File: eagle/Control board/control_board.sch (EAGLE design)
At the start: 179 parts, among them SW1 SPST_TACT-EVQQ2, SW2 SPST_TACT-EVQQ2, U1 TCA9554A, U2 LM317, U3 LM317, U4 STM32F446, U5 TCA9554A, U6 TCA9554A, X1 JST-XH-02-PIN-LONG-PAD, X10 JST-XH-07-PIN-LONG-PAD, X11 JST-XH-07-PIN-LONG-PAD, X12 JST-XH-02-PIN-LONG-PAD, X13 JST-XH-03-PIN-LONG-PAD, X14 JST-XH-03-PIN-LONG-PAD, X15 JST-XH-08-PIN-LONG-PAD, X16 JST-XH-02-PIN-LONG-PAD, X17 JST-XH-08-PIN-LONG-PAD, X18 JST-XH-02-PIN-LONG-PAD, X2 JST-XH-06-PIN-LONG-PAD, X3 JST-XH-06-PIN-LONG-PAD, X4 JST-XH-06-PIN-LONG-PAD, X5 JST-XH-06-PIN-LONG-PAD, X6 JST-XH-06-PIN-LONG-PAD, X7 JST-XH-06-PIN-LONG-PAD, X8 JST-XH-04-PIN-LONG-PAD, X9 JST-XH-07-PIN-LONG-PAD

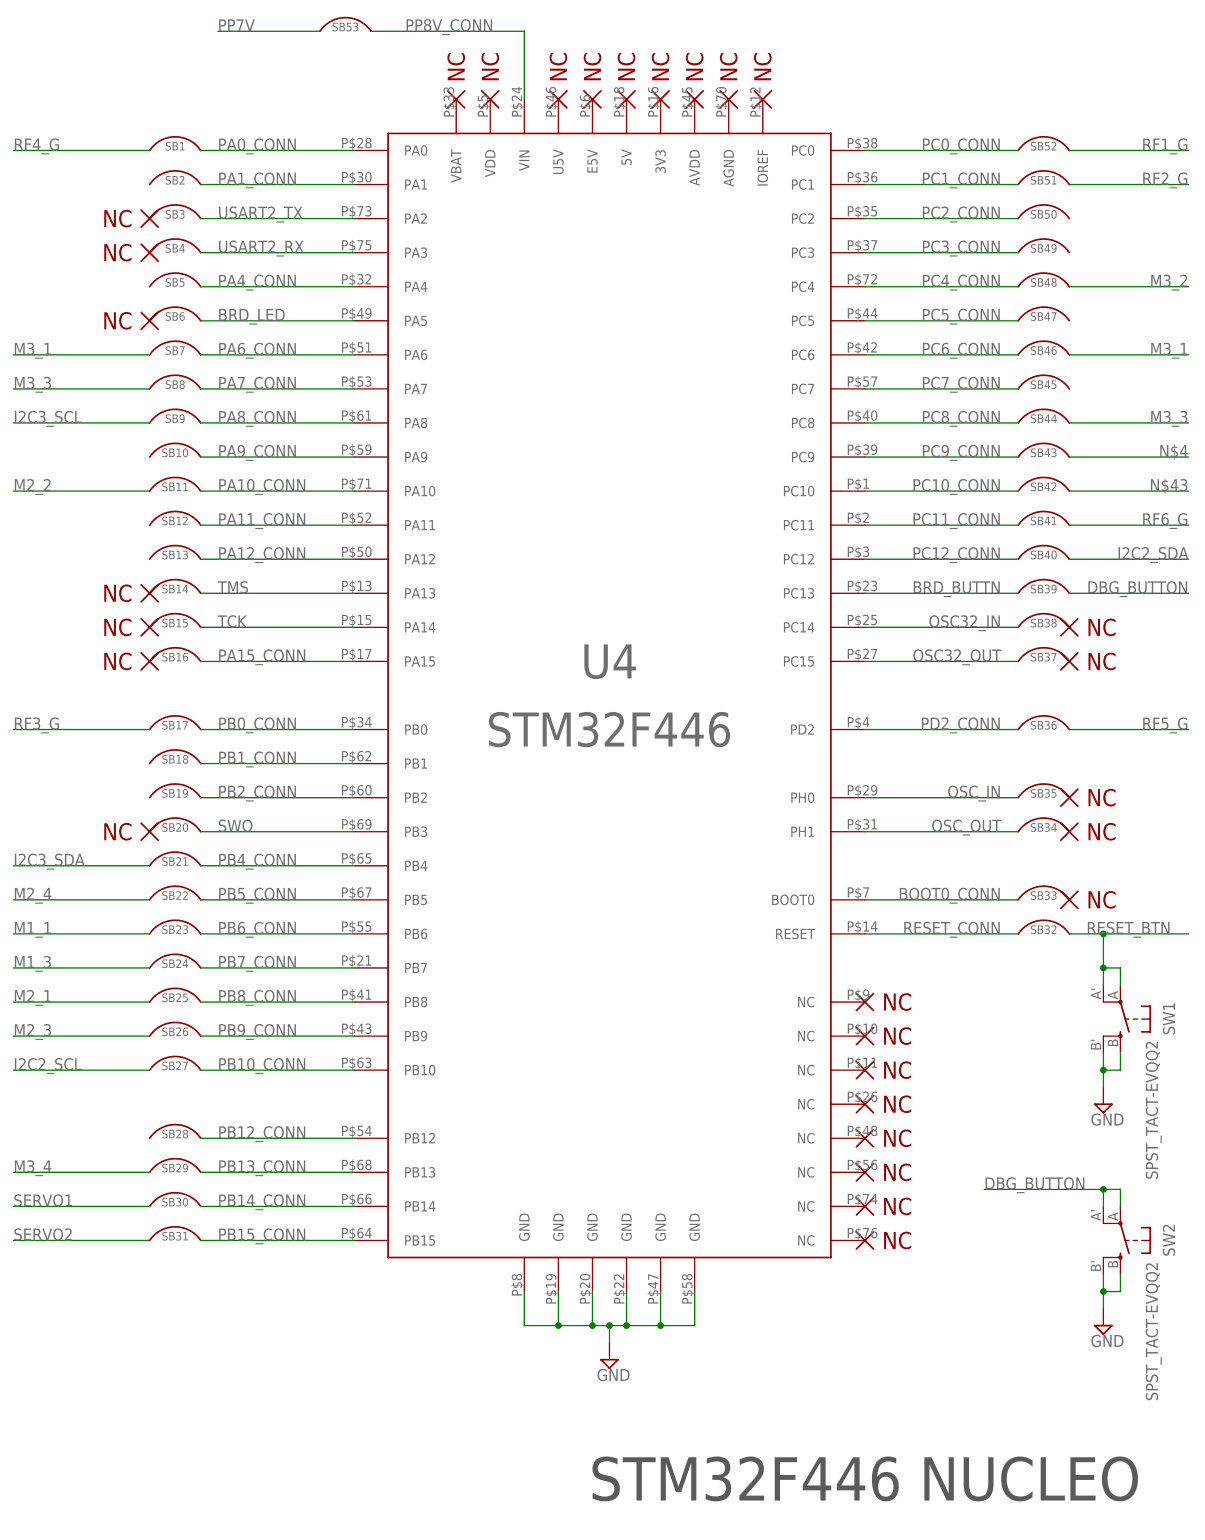
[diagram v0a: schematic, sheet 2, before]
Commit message: Nearly done assigning gpio
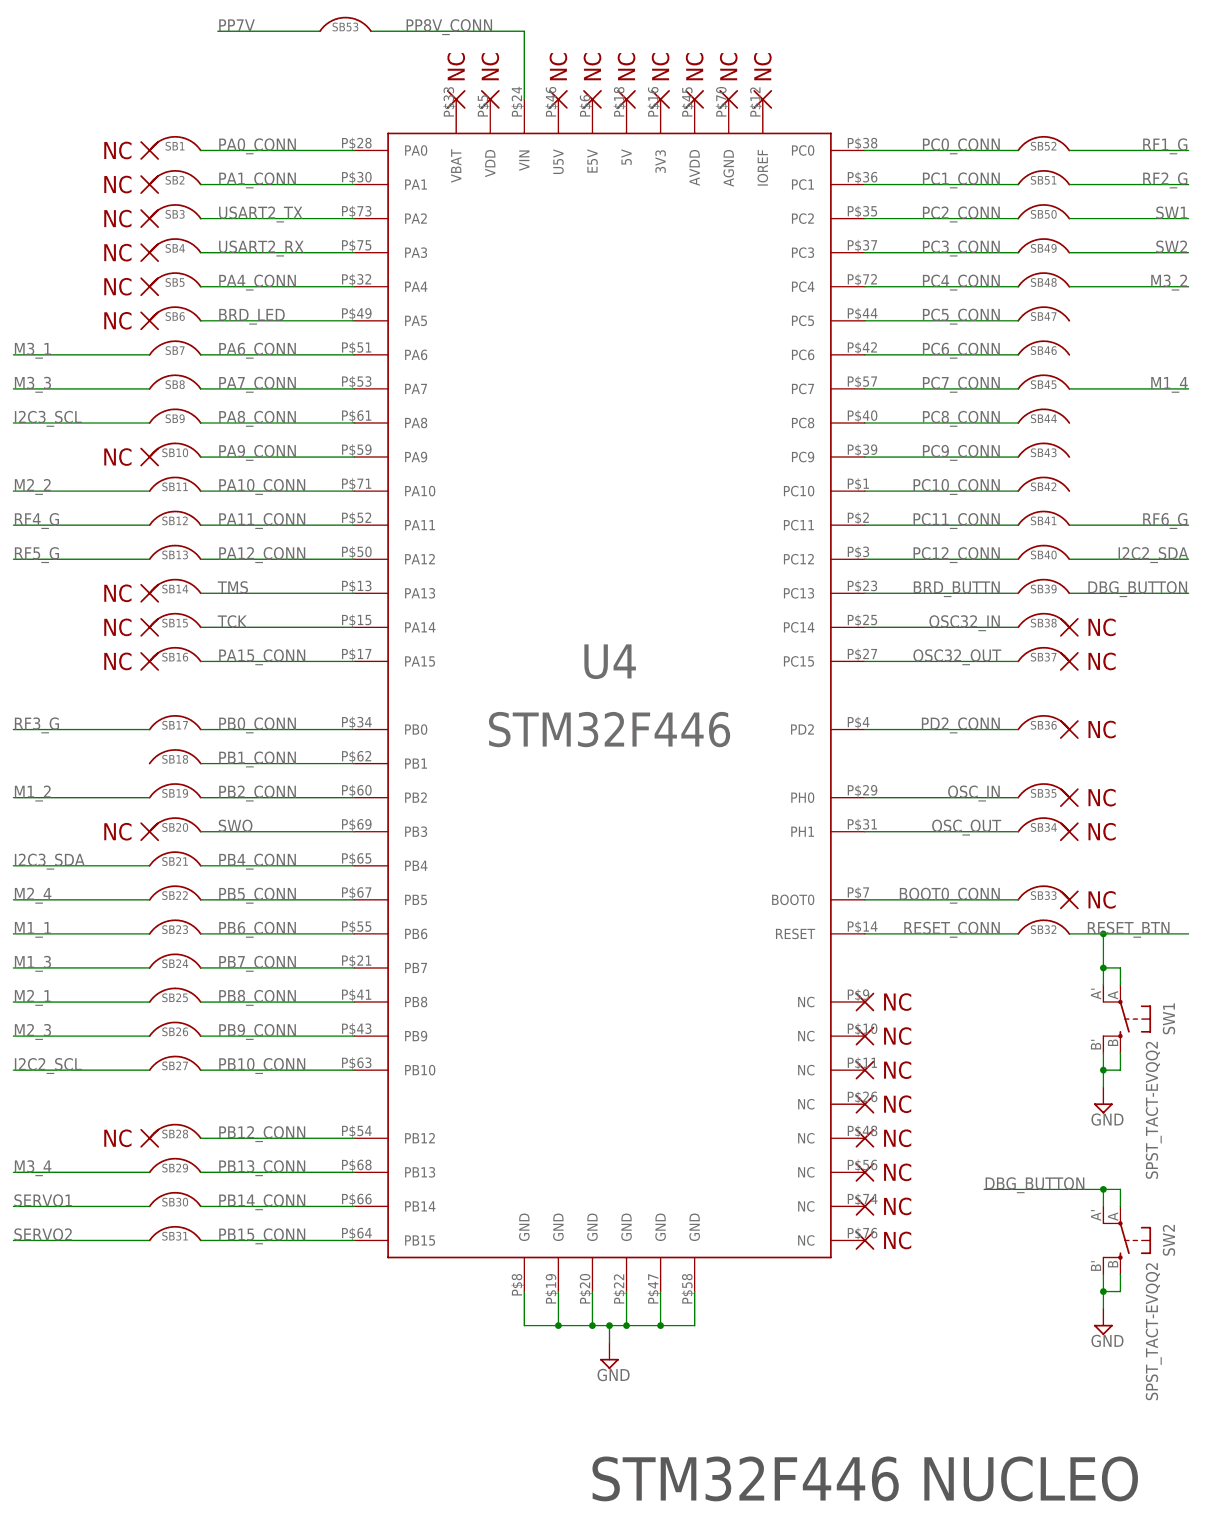
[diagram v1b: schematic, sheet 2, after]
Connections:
- removed net N$4: SB43.P$1
- removed net N$43: SB42.P$2
- net M1_2: now also SB19.P$1
- net M1_4: now also SB45.P$1
- net M3_1: no longer SB46.P$2
- net M3_3: no longer SB44.P$2
- net RF4_G: now also SB12.P$1; no longer SB1.P$1
- net RF5_G: now also SB13.P$1; no longer SB36.P$2
- net SW1: now also SB50.P$2
- net SW2: now also SB49.P$2
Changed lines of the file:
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@@
 <part name="R11" library="rcl" deviceset="R-US_" device="R0603" value="100"/>
 <part name="R12" library="rcl" deviceset="R-US_" device="R0603" value="100"/>
+<part name="U$27" library="custom" deviceset="NC" device=""/>
+<part name="U$34" library="custom" deviceset="NC" device=""/>
+<part name="U$35" library="custom" deviceset="NC" device=""/>
+<part name="U$36" library="custom" deviceset="NC" device=""/>
+<part name="U$38" library="custom" deviceset="NC" device=""/>
+<part name="U$39" library="custom" deviceset="NC" device=""/>
 </parts>
 <sheets>
@@
 <attribute name="DIGI" x="167.64" y="63.5" size="1.778" layer="96" rot="R180" display="off"/>
 </instance>
+<instance part="U$27" gate="G$1" x="22.86" y="180.34" rot="R180"/>
+<instance part="U$34" gate="G$1" x="160.02" y="139.7"/>
+<instance part="U$35" gate="G$1" x="22.86" y="226.06" rot="R180"/>
+<instance part="U$36" gate="G$1" x="22.86" y="220.98" rot="R180"/>
+<instance part="U$38" gate="G$1" x="22.86" y="78.74" rot="R180"/>
+<instance part="U$39" gate="G$1" x="22.86" y="205.74" rot="R180"/>
 </instances>
 <busses>
@@
 <net name="M3_1" class="0">
 <segment>
-<pinref part="SB46" gate="G$1" pin="P$2"/>
-<wire x1="160.02" y1="195.58" x2="177.8" y2="195.58" width="0.1524" layer="91"/>
-<label x="177.8" y="195.58" size="1.778" layer="95" rot="MR0"/>
-</segment>
-<segment>
 <pinref part="SB7" gate="G$1" pin="P$1"/>
 <wire x1="22.86" y1="195.58" x2="2.54" y2="195.58" width="0.1524" layer="91"/>
@@
 <net name="M3_3" class="0">
 <segment>
-<pinref part="SB44" gate="G$1" pin="P$2"/>
-<wire x1="160.02" y1="185.42" x2="177.8" y2="185.42" width="0.1524" layer="91"/>
-<label x="177.8" y="185.42" size="1.778" layer="95" rot="MR0"/>
-</segment>
-<segment>
 <pinref part="SB8" gate="G$1" pin="P$1"/>
 <wire x1="22.86" y1="190.5" x2="2.54" y2="190.5" width="0.1524" layer="91"/>
 <label x="2.54" y="190.5" size="1.778" layer="95"/>
-</segment>
-</net>
-<net name="N$43" class="0">
-<segment>
-<pinref part="SB42" gate="G$1" pin="P$2"/>
-<wire x1="160.02" y1="175.26" x2="177.8" y2="175.26" width="0.1524" layer="91"/>
-<label x="177.8" y="175.26" size="1.778" layer="95" rot="MR0"/>
 </segment>
 </net>
@@
 </segment>
 </net>
-<net name="N$4" class="0">
-<segment>
-<pinref part="SB43" gate="G$1" pin="P$1"/>
-<wire x1="160.02" y1="180.34" x2="177.8" y2="180.34" width="0.1524" layer="91"/>
-<label x="177.8" y="180.34" size="1.778" layer="95" rot="MR0"/>
-</segment>
-</net>
 <net name="M2_1" class="0">
 <segment>
@@
 </segment>
 </net>
-<net name="RF4_G" class="0">
-<segment>
-<pinref part="SB1" gate="G$1" pin="P$1"/>
-<wire x1="22.86" y1="226.06" x2="2.54" y2="226.06" width="0.1524" layer="91"/>
-<label x="2.54" y="226.06" size="1.778" layer="95"/>
-</segment>
-</net>
 <net name="RF3_G" class="0">
 <segment>
@@
 </segment>
 </net>
-<net name="RF5_G" class="0">
-<segment>
-<pinref part="SB36" gate="G$1" pin="P$2"/>
-<wire x1="160.02" y1="139.7" x2="177.8" y2="139.7" width="0.1524" layer="91"/>
-<label x="177.8" y="139.7" size="1.778" layer="95" rot="MR0"/>
-</segment>
-</net>
 <net name="M3_2" class="0">
 <segment>
@@
 </segment>
 </net>
+<net name="M1_4" class="0">
+<segment>
+<pinref part="SB45" gate="G$1" pin="P$1"/>
+<wire x1="160.02" y1="190.5" x2="177.8" y2="190.5" width="0.1524" layer="91"/>
+<label x="177.8" y="190.5" size="1.778" layer="95" rot="MR0"/>
+</segment>
+</net>
+<net name="SW1" class="0">
+<segment>
+<pinref part="SB50" gate="G$1" pin="P$2"/>
+<wire x1="160.02" y1="215.9" x2="177.8" y2="215.9" width="0.1524" layer="91"/>
+<label x="177.8" y="215.9" size="1.778" layer="95" rot="MR0"/>
+</segment>
+</net>
+<net name="SW2" class="0">
+<segment>
+<pinref part="SB49" gate="G$1" pin="P$2"/>
+<wire x1="177.8" y1="210.82" x2="160.02" y2="210.82" width="0.1524" layer="91"/>
+<label x="177.8" y="210.82" size="1.778" layer="95" rot="MR0"/>
+</segment>
+</net>
+<net name="M1_2" class="0">
+<segment>
+<pinref part="SB19" gate="G$1" pin="P$1"/>
+<wire x1="22.86" y1="129.54" x2="2.54" y2="129.54" width="0.1524" layer="91"/>
+<label x="2.54" y="129.54" size="1.778" layer="95"/>
+</segment>
+</net>
+<net name="RF4_G" class="0">
+<segment>
+<pinref part="SB12" gate="G$1" pin="P$1"/>
+<wire x1="22.86" y1="170.18" x2="2.54" y2="170.18" width="0.1524" layer="91"/>
+<label x="2.54" y="170.18" size="1.778" layer="95"/>
+</segment>
+</net>
+<net name="RF5_G" class="0">
+<segment>
+<pinref part="SB13" gate="G$1" pin="P$1"/>
+<wire x1="2.54" y1="165.1" x2="22.86" y2="165.1" width="0.1524" layer="91"/>
+<label x="2.54" y="165.1" size="1.778" layer="95"/>
+</segment>
+</net>
